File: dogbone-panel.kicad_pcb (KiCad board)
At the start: 2 copper layers, 26.6 x 63.3 mm, 176 parts, among them M1 THRU_HOLE_PAD, M10 THRU_HOLE_PAD, M11 THRU_HOLE_PAD, M12 THRU_HOLE_PAD, M2 THRU_HOLE_PAD, M3 THRU_HOLE_PAD, M4 THRU_HOLE_PAD, M5 THRU_HOLE_PAD, M6 THRU_HOLE_PAD, M7 THRU_HOLE_PAD, M8 THRU_HOLE_PAD, M9 THRU_HOLE_PAD

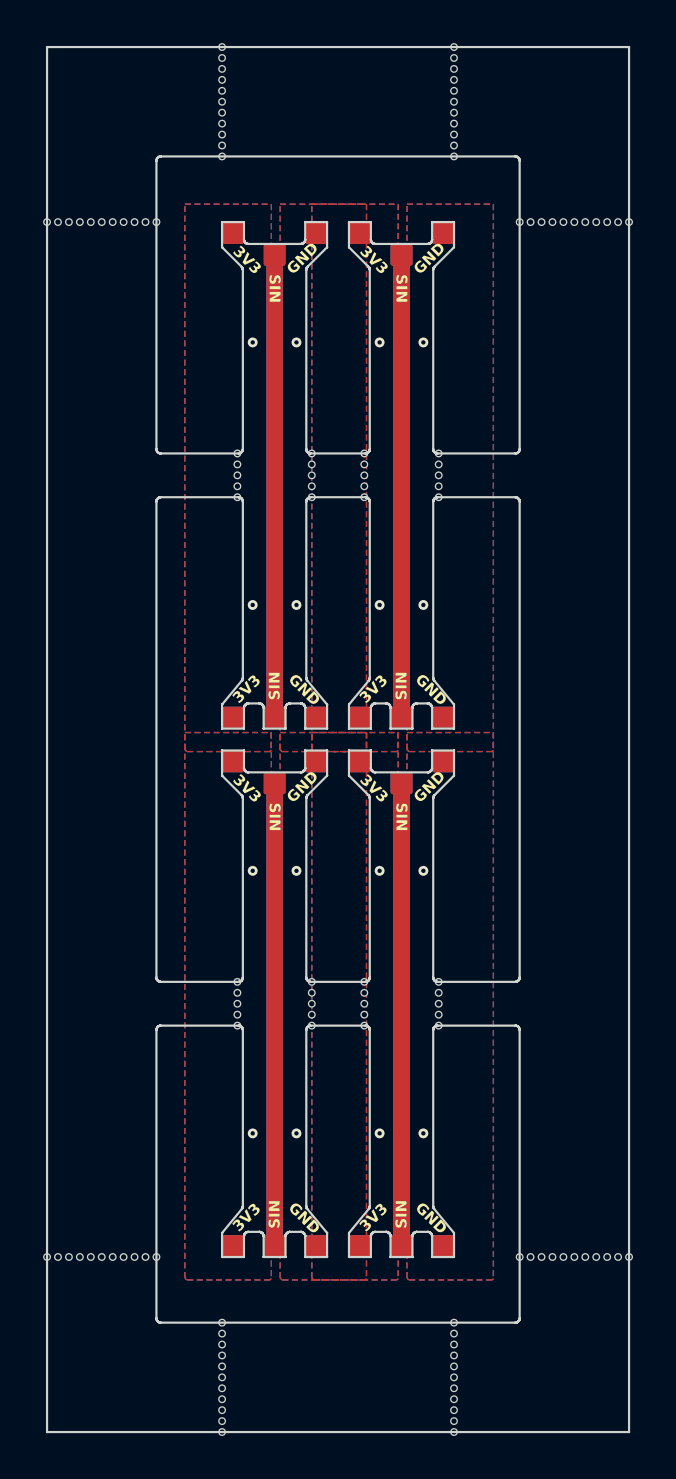
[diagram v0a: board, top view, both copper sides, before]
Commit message: panelization options
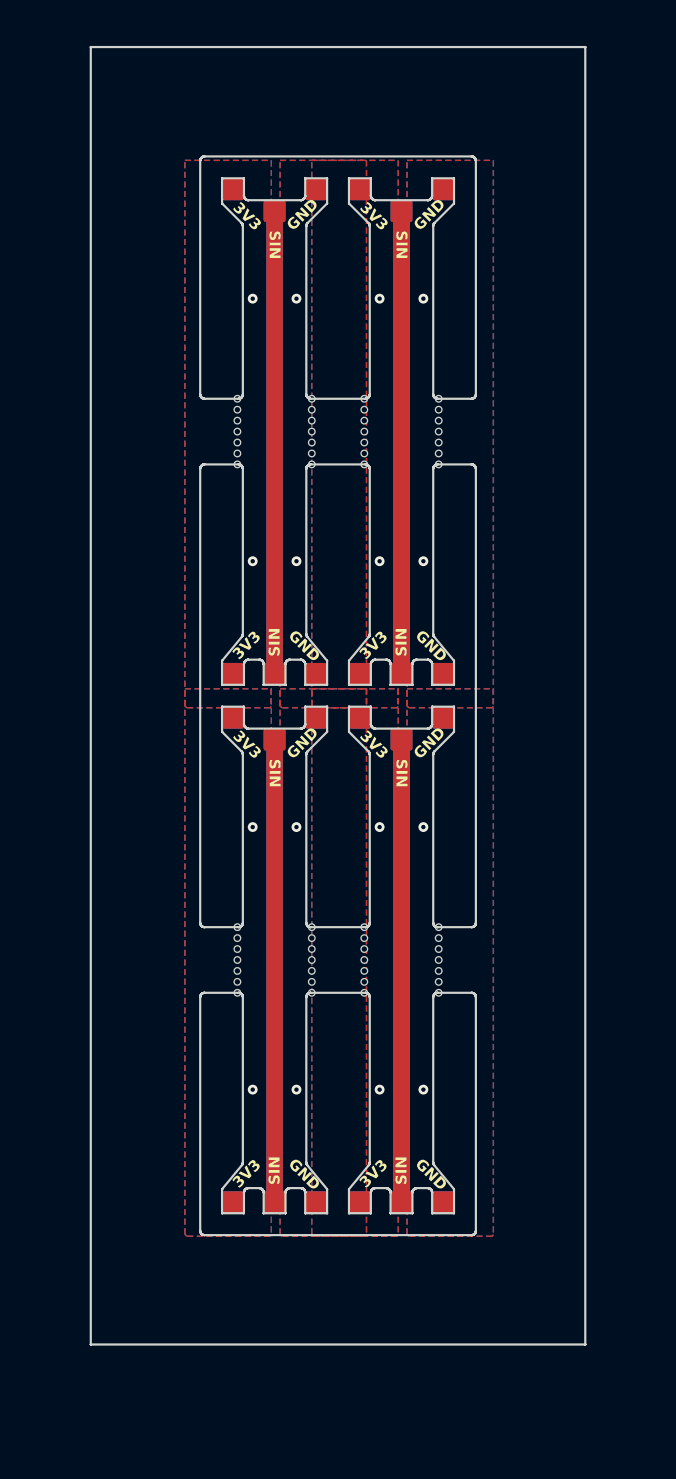
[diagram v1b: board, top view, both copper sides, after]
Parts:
- removed KiKit_MB_10_10, KiKit_MB_10_11, KiKit_MB_10_12, KiKit_MB_10_2, KiKit_MB_10_3, KiKit_MB_10_4, KiKit_MB_10_5, KiKit_MB_10_6, KiKit_MB_10_7, KiKit_MB_10_8, KiKit_MB_10_9, KiKit_MB_11_10, KiKit_MB_11_11, KiKit_MB_11_12, KiKit_MB_11_2, KiKit_MB_11_3, KiKit_MB_11_4, KiKit_MB_11_5, KiKit_MB_11_6, KiKit_MB_11_7, KiKit_MB_11_8, KiKit_MB_11_9, KiKit_MB_12_10, KiKit_MB_12_11, KiKit_MB_12_12, KiKit_MB_12_2, KiKit_MB_12_3, KiKit_MB_12_4, KiKit_MB_12_5, KiKit_MB_12_6, KiKit_MB_12_7, KiKit_MB_12_8, KiKit_MB_12_9, KiKit_MB_13_10, KiKit_MB_13_11, KiKit_MB_13_12, KiKit_MB_13_2, KiKit_MB_13_3, KiKit_MB_13_4, KiKit_MB_13_5, KiKit_MB_13_6, KiKit_MB_13_7, KiKit_MB_13_8, KiKit_MB_13_9, KiKit_MB_14_10, KiKit_MB_14_11, KiKit_MB_14_12, KiKit_MB_14_2, KiKit_MB_14_3, KiKit_MB_14_4, KiKit_MB_14_5, KiKit_MB_14_6, KiKit_MB_14_7, KiKit_MB_14_8, KiKit_MB_14_9, KiKit_MB_15_10, KiKit_MB_15_11, KiKit_MB_15_12, KiKit_MB_15_2, KiKit_MB_15_3, KiKit_MB_15_4, KiKit_MB_15_5, KiKit_MB_15_6, KiKit_MB_15_7, KiKit_MB_15_8, KiKit_MB_15_9, KiKit_MB_16_10, KiKit_MB_16_11, KiKit_MB_16_12, KiKit_MB_16_2, KiKit_MB_16_3, KiKit_MB_16_4, KiKit_MB_16_5, KiKit_MB_16_6, KiKit_MB_16_7, KiKit_MB_16_8, KiKit_MB_16_9, KiKit_MB_9_10, KiKit_MB_9_11, KiKit_MB_9_12, KiKit_MB_9_2, KiKit_MB_9_3, KiKit_MB_9_4, KiKit_MB_9_5, KiKit_MB_9_6, KiKit_MB_9_7, KiKit_MB_9_8, KiKit_MB_9_9: NPTH, NPTH
- removed the M1 at (143.7, 52.6)
- removed the M1 at (149.5, 28.5)
- removed the M1 at (143.7, 28.5)
- removed the M1 at (149.5, 52.6)
- removed the M10 at (149.5, 74.8)
- removed the M10 at (143.7, 50.6)
- removed the M10 at (149.5, 50.6)
- removed the M10 at (143.7, 74.8)
- removed the M11 at (147.5, 50.6)
- removed the M11 at (147.5, 74.8)
- removed the M11 at (153.3, 74.8)
- removed the M11 at (153.3, 50.6)
- removed the M12 at (153.3, 74.8)
- removed the M12 at (153.3, 50.6)
- removed the M12 at (147.5, 74.8)
- removed the M12 at (147.5, 50.6)
- removed the M2 at (145.6, 50.6)
- removed the M2 at (151.4, 74.8)
- removed the M2 at (151.4, 50.6)
- removed the M2 at (145.6, 74.8)
- removed the M3 at (143.7, 50.6)
- removed the M3 at (149.5, 50.6)
- removed the M3 at (149.5, 74.8)
- removed the M3 at (143.7, 74.8)
- removed the M4 at (151.4, 53.6)
- removed the M4 at (145.6, 29.5)
- removed the M4 at (145.6, 53.6)
- removed the M4 at (151.4, 29.5)
- removed the M5 at (147.5, 28.5)
- removed the M5 at (147.5, 52.6)
- removed the M5 at (153.3, 52.6)
- removed the M5 at (153.3, 28.5)
- removed the M6 at (145.6, 50.6)
- removed the M6 at (151.4, 74.8)
- removed the M6 at (145.6, 74.8)
- removed the M6 at (151.4, 50.6)
- removed the M7 at (153.3, 28.5)
- removed the M7 at (147.5, 28.5)
- removed the M7 at (147.5, 52.6)
- removed the M7 at (153.3, 52.6)
- removed the M8 at (145.6, 29.5)
- removed the M8 at (151.4, 29.5)
- removed the M8 at (145.6, 53.6)
- removed the M8 at (151.4, 53.6)
- removed the M9 at (143.7, 52.6)
- removed the M9 at (143.7, 28.5)
- removed the M9 at (149.5, 28.5)
- removed the M9 at (149.5, 52.6)
- added KiKit_MB_1_7: NPTH, NPTH, F.Cu at (143.9, 36.6)
- added KiKit_MB_1_8: NPTH, NPTH, F.Cu at (143.9, 36.1)
- added KiKit_MB_2_7: NPTH, NPTH, F.Cu at (147.3, 38.6)
- added KiKit_MB_2_8: NPTH, NPTH, F.Cu at (147.3, 39.1)
- added KiKit_MB_3_7: NPTH, NPTH, F.Cu at (149.7, 36.6)
- added KiKit_MB_3_8: NPTH, NPTH, F.Cu at (149.7, 36.1)
- added KiKit_MB_4_7: NPTH, NPTH, F.Cu at (153.1, 38.6)
- added KiKit_MB_4_8: NPTH, NPTH, F.Cu at (153.1, 39.1)
- added KiKit_MB_5_7: NPTH, NPTH, F.Cu at (143.9, 60.7)
- added KiKit_MB_5_8: NPTH, NPTH, F.Cu at (143.9, 60.2)
- added KiKit_MB_6_7: NPTH, NPTH, F.Cu at (147.3, 62.7)
- added KiKit_MB_6_8: NPTH, NPTH, F.Cu at (147.3, 63.2)
- added KiKit_MB_7_7: NPTH, NPTH, F.Cu at (149.7, 60.7)
- added KiKit_MB_7_8: NPTH, NPTH, F.Cu at (149.7, 60.2)
- added KiKit_MB_8_7: NPTH, NPTH, F.Cu at (153.1, 62.7)
- added KiKit_MB_8_8: NPTH, NPTH, F.Cu at (153.1, 63.2)
- added M1: THRU_HOLE_PAD, adapter-encoder:dogbone_pad, F.Cu at (149.5, 26.5)
- added M1: THRU_HOLE_PAD, adapter-encoder:dogbone_pad, F.Cu at (143.7, 26.5)
- added M1: THRU_HOLE_PAD, adapter-encoder:dogbone_pad, F.Cu at (143.7, 50.6)
- added M1: THRU_HOLE_PAD, adapter-encoder:dogbone_pad, F.Cu at (149.5, 50.6)
- added M10: THRU_HOLE_PAD, adapter-encoder:dogbone_pad, B.Cu at (149.5, 48.6)
- added M10: THRU_HOLE_PAD, adapter-encoder:dogbone_pad, B.Cu at (143.7, 48.6)
- added M10: THRU_HOLE_PAD, adapter-encoder:dogbone_pad, B.Cu at (149.5, 72.8)
- added M10: THRU_HOLE_PAD, adapter-encoder:dogbone_pad, B.Cu at (143.7, 72.8)
- added M11: THRU_HOLE_PAD, adapter-encoder:dogbone_pad, F.Cu at (153.3, 72.8)
- added M11: THRU_HOLE_PAD, adapter-encoder:dogbone_pad, F.Cu at (147.5, 72.8)
- added M11: THRU_HOLE_PAD, adapter-encoder:dogbone_pad, F.Cu at (147.5, 48.6)
- added M11: THRU_HOLE_PAD, adapter-encoder:dogbone_pad, F.Cu at (153.3, 48.6)
- added M12: THRU_HOLE_PAD, adapter-encoder:dogbone_pad, B.Cu at (153.3, 48.6)
- added M12: THRU_HOLE_PAD, adapter-encoder:dogbone_pad, B.Cu at (147.5, 48.6)
- added M12: THRU_HOLE_PAD, adapter-encoder:dogbone_pad, B.Cu at (153.3, 72.8)
- added M12: THRU_HOLE_PAD, adapter-encoder:dogbone_pad, B.Cu at (147.5, 72.8)
- added M2: THRU_HOLE_PAD, adapter-encoder:dogbone_pad, F.Cu at (145.6, 48.6)
- added M2: THRU_HOLE_PAD, adapter-encoder:dogbone_pad, F.Cu at (151.4, 48.6)
- added M2: THRU_HOLE_PAD, adapter-encoder:dogbone_pad, F.Cu at (145.6, 72.8)
- added M2: THRU_HOLE_PAD, adapter-encoder:dogbone_pad, F.Cu at (151.4, 72.8)
- added M3: THRU_HOLE_PAD, adapter-encoder:dogbone_pad, F.Cu at (143.7, 72.8)
- added M3: THRU_HOLE_PAD, adapter-encoder:dogbone_pad, F.Cu at (143.7, 48.6)
- added M3: THRU_HOLE_PAD, adapter-encoder:dogbone_pad, F.Cu at (149.5, 48.6)
- added M3: THRU_HOLE_PAD, adapter-encoder:dogbone_pad, F.Cu at (149.5, 72.8)
- added M4: THRU_HOLE_PAD, adapter-encoder:dogbone_pad, F.Cu at (151.4, 51.6)
- added M4: THRU_HOLE_PAD, adapter-encoder:dogbone_pad, F.Cu at (145.6, 51.6)
- added M4: THRU_HOLE_PAD, adapter-encoder:dogbone_pad, F.Cu at (151.4, 27.5)
- added M4: THRU_HOLE_PAD, adapter-encoder:dogbone_pad, F.Cu at (145.6, 27.5)
- added M5: THRU_HOLE_PAD, adapter-encoder:dogbone_pad, F.Cu at (153.3, 26.5)
- added M5: THRU_HOLE_PAD, adapter-encoder:dogbone_pad, F.Cu at (147.5, 26.5)
- added M5: THRU_HOLE_PAD, adapter-encoder:dogbone_pad, F.Cu at (147.5, 50.6)
- added M5: THRU_HOLE_PAD, adapter-encoder:dogbone_pad, F.Cu at (153.3, 50.6)
- added M6: THRU_HOLE_PAD, adapter-encoder:dogbone_pad, B.Cu at (145.6, 72.8)
- added M6: THRU_HOLE_PAD, adapter-encoder:dogbone_pad, B.Cu at (151.4, 72.8)
- added M6: THRU_HOLE_PAD, adapter-encoder:dogbone_pad, B.Cu at (151.4, 48.6)
- added M6: THRU_HOLE_PAD, adapter-encoder:dogbone_pad, B.Cu at (145.6, 48.6)
- added M7: THRU_HOLE_PAD, adapter-encoder:dogbone_pad, B.Cu at (153.3, 50.6)
- added M7: THRU_HOLE_PAD, adapter-encoder:dogbone_pad, B.Cu at (147.5, 26.5)
- added M7: THRU_HOLE_PAD, adapter-encoder:dogbone_pad, B.Cu at (153.3, 26.5)
- added M7: THRU_HOLE_PAD, adapter-encoder:dogbone_pad, B.Cu at (147.5, 50.6)
- added M8: THRU_HOLE_PAD, adapter-encoder:dogbone_pad, B.Cu at (145.6, 27.5)
- added M8: THRU_HOLE_PAD, adapter-encoder:dogbone_pad, B.Cu at (151.4, 51.6)
- added M8: THRU_HOLE_PAD, adapter-encoder:dogbone_pad, B.Cu at (151.4, 27.5)
- added M8: THRU_HOLE_PAD, adapter-encoder:dogbone_pad, B.Cu at (145.6, 51.6)
- added M9: THRU_HOLE_PAD, adapter-encoder:dogbone_pad, B.Cu at (143.7, 26.5)
- added M9: THRU_HOLE_PAD, adapter-encoder:dogbone_pad, B.Cu at (149.5, 26.5)
- added M9: THRU_HOLE_PAD, adapter-encoder:dogbone_pad, B.Cu at (149.5, 50.6)
- added M9: THRU_HOLE_PAD, adapter-encoder:dogbone_pad, B.Cu at (143.7, 50.6)
- moved KiKit_MB_2_2 2.50 mm to (147.3, 36.1)
- moved KiKit_MB_2_3 2.50 mm to (147.3, 36.6)
- moved KiKit_MB_2_4 2.50 mm to (147.3, 37.1)
- moved KiKit_MB_2_5 2.50 mm to (147.3, 37.6)
- moved KiKit_MB_2_6 2.50 mm to (147.3, 38.1)
- moved KiKit_MB_4_2 2.50 mm to (153.1, 36.1)
- moved KiKit_MB_4_3 2.50 mm to (153.1, 36.6)
- moved KiKit_MB_4_4 2.50 mm to (153.1, 37.1)
- moved KiKit_MB_4_5 2.50 mm to (153.1, 37.6)
- moved KiKit_MB_4_6 2.50 mm to (153.1, 38.1)
- moved KiKit_MB_6_2 2.50 mm to (147.3, 60.2)
- moved KiKit_MB_6_3 2.50 mm to (147.3, 60.7)
- moved KiKit_MB_6_4 2.50 mm to (147.3, 61.2)
- moved KiKit_MB_8_2 2.50 mm to (153.1, 60.2)
- moved KiKit_MB_8_3 2.50 mm to (153.1, 60.7)
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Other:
- board size 26.6 x 63.3 mm -> 22.6 x 59.3 mm
